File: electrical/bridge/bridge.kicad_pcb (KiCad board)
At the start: 2 copper layers, 42.2 x 24.2 mm, 28 parts, among them J1 USB_OTG, J2 USB_A, J3 swd, P1 ~rst~, P2 bootldr, U1 crystal-4pin, U2 stm32f405rgt6, U3 my-NCP1117ST50T3G

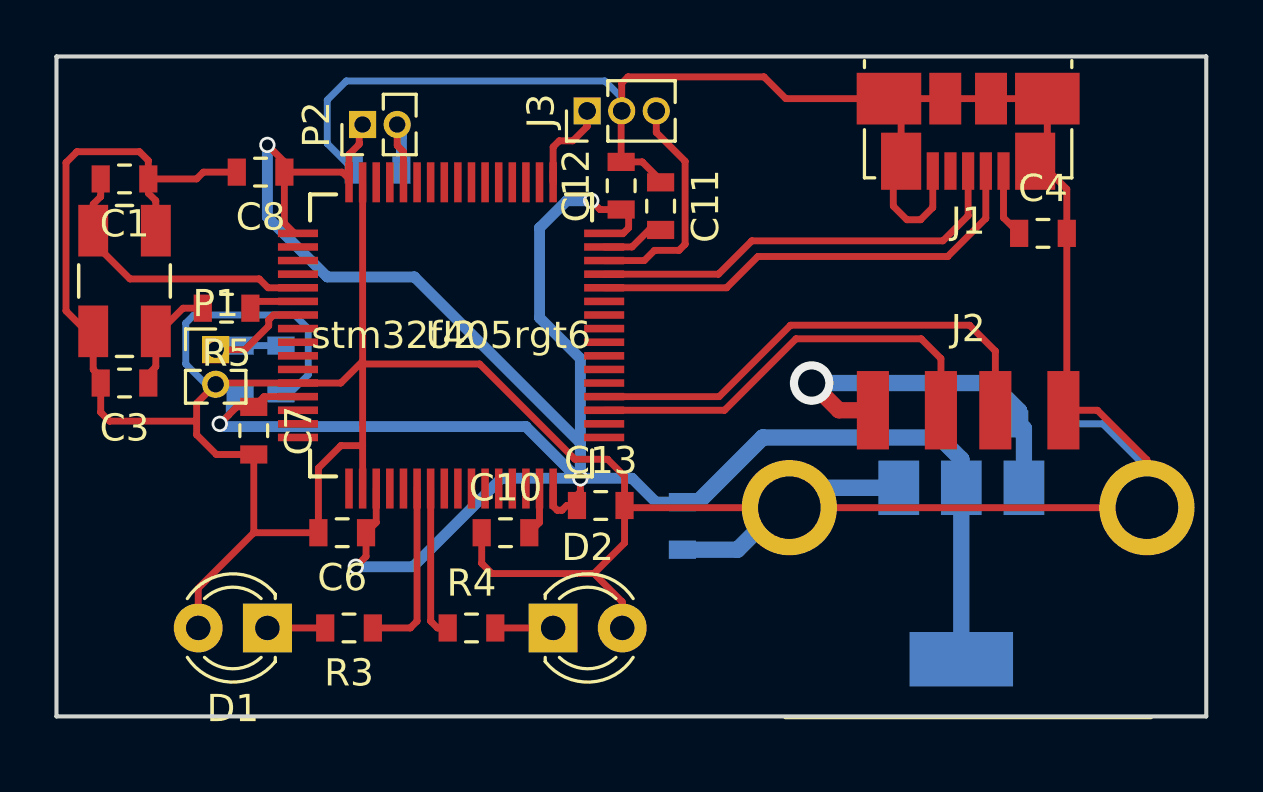
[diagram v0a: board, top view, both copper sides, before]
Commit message: Done with routing.
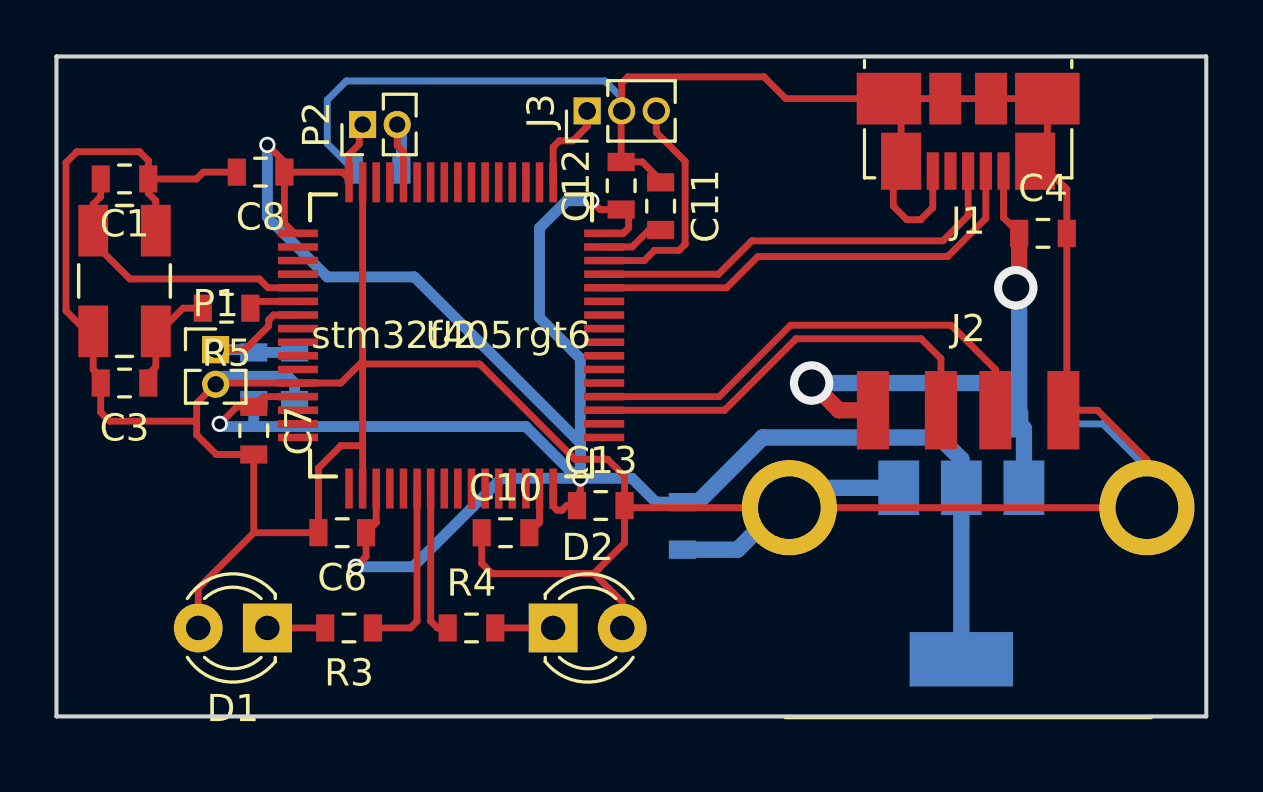
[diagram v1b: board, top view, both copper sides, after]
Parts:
- moved C2 0.56 mm to (157.5, 99.2)
- moved R2 0.56 mm to (156.0, 99.2)
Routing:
- net /vbus: track 16.1 -> 23.2 mm, vias 1 -> 2
- net GND: track 187.6 -> 180.6 mm
- added copper zone on F.Cu, net GND
- added copper zone on B.Cu, net VDD
